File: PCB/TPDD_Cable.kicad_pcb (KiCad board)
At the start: 2 copper layers, 10.4 x 14.5 mm, 5 parts, among them J1 Wire Solder Pads, J2 TPDD, Q1 DTA114EKA, Q2 DTA114EKA, Q3 DTA114EKA

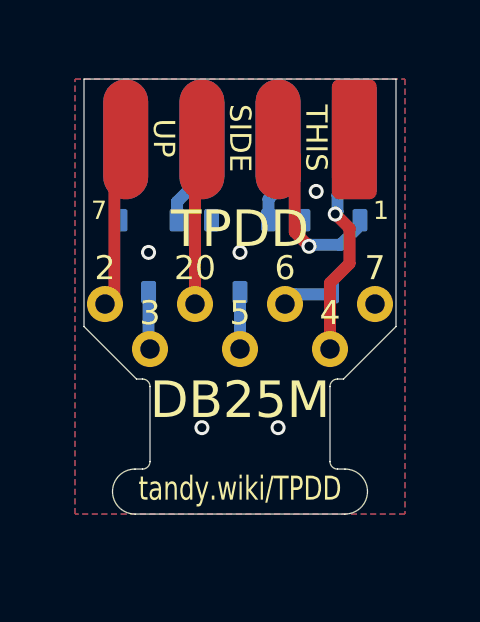
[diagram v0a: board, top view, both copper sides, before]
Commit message: pcb shape v012
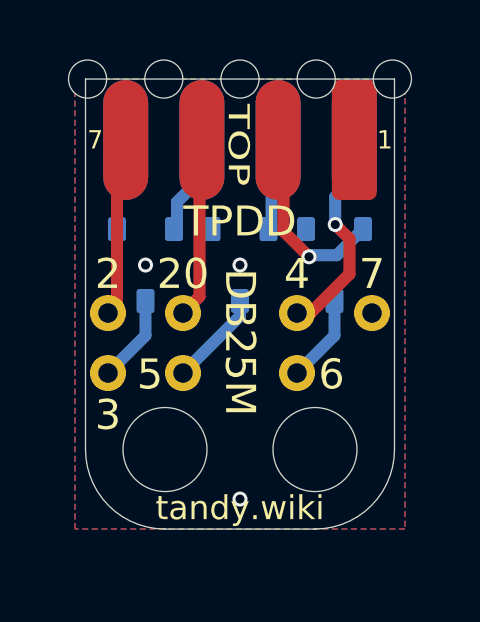
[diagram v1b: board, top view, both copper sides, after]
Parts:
- added REF**: npth_m3, 000_LOCAL:npth_m3, F.Cu at (147.5, 92.0)
- added REF**: npth_m3, 000_LOCAL:npth_m3, F.Cu at (142.5, 92.0)
- moved J2 4.31 mm to (145.0, 79.6)
- moved J1 0.35 mm to (145.0, 88.2)
- moved Q1 0.31 mm to (148.1, 85.8)
- moved Q3 0.31 mm to (141.8, 85.8)
- moved Q2 0.30 mm to (145.0, 85.8)
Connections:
- J1 pad 5: /DSR -> /RTS
- J1 pad 6: /RTS -> /DSR
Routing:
- net /CTS: track 1.89 -> 3.19 mm
- net /DSR: track 1.71 -> 2.92 mm
- net /RX: track 1.91 -> 2.92 mm
- net /RTS: track 7.72 -> 7.22 mm
- net /SG: vias 5 -> 3
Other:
- board size 10.4 x 14.5 mm -> 10.3 x 15 mm
- board text added: "${00000000-0000-0000-0000-00005d2d4345:VALUE}"
- board text added: "BOTTOM"
- board text added: "TOP"
- board text added: "tandy.wiki"
- board text removed: "DOWN"
- board text removed: "Q1,Q2,Q3 ${00000000-0000-0000-0000-00005d2d4345:VALUE}"
- board text removed: "SIDE"
- board text removed: "THIS"
- board text removed: "UP"
- board text removed: "tandy.wiki/TPDD"

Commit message: pcb version 3
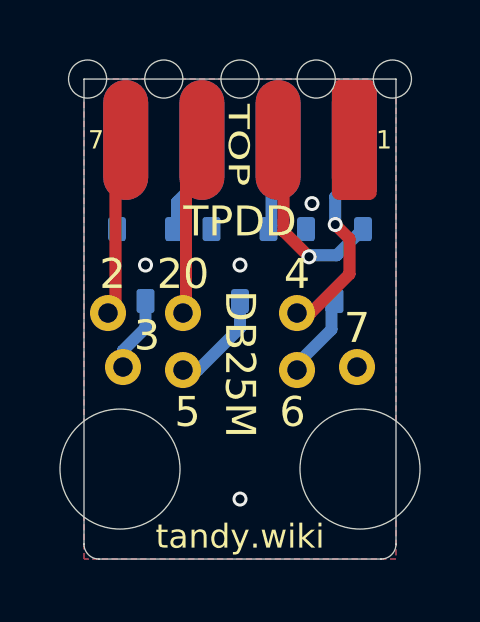
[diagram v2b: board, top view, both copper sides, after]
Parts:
- removed J1: Wire Solder Pads, 000_LOCAL:D7_1.5mm_wirepads
- added P2: RX, 000_LOCAL:PTH_0.65x1.2, F.Cu at (140.6, 87.4)
- added P20: DSR, 000_LOCAL:PTH_0.65x1.2, F.Cu at (143.1, 87.4)
- added P3: TX, 000_LOCAL:PTH_0.65x1.2, F.Cu at (141.1, 89.2)
- added P4: CTS, 000_LOCAL:PTH_0.65x1.2, F.Cu at (146.9, 89.3)
- added P5: RTS, 000_LOCAL:PTH_0.65x1.2, F.Cu at (143.1, 89.3)
- added P6: DTR, 000_LOCAL:PTH_0.65x1.2, F.Cu at (146.9, 87.4)
- added P7: GND, 000_LOCAL:PTH_0.65x1.2, F.Cu at (148.9, 89.2)
- moved REF** 1.63 mm to (149.0, 92.6)
- moved REF** 1.63 mm to (141.0, 92.6)
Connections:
- net /SG renamed GND
- J2 pad 8: (no net) -> /EB+
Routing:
- net GND: vias 3 -> 4
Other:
- board size 10.3 x 15 mm -> 10.4 x 16 mm
